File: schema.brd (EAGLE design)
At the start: 59.4 x 55.9 mm, 24 parts, among them Q1 2N2907

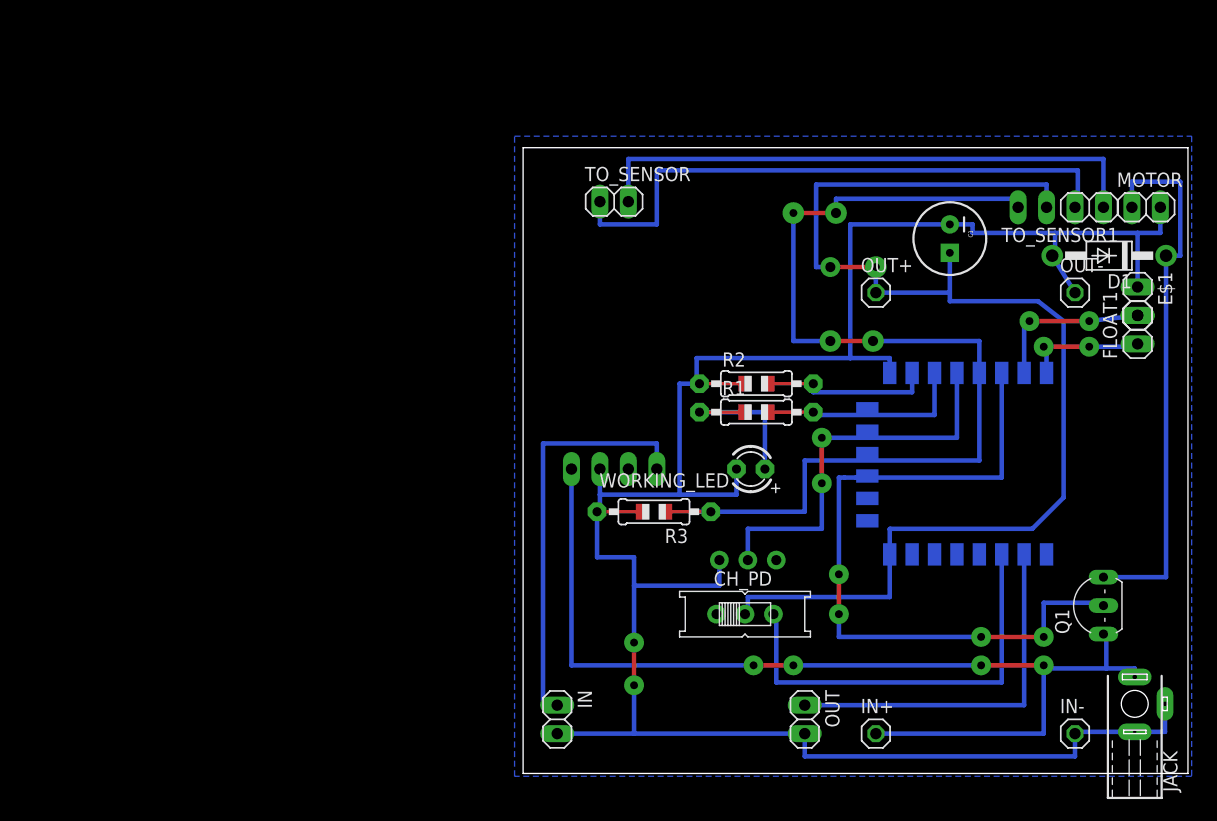
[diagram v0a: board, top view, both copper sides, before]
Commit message: Version 2
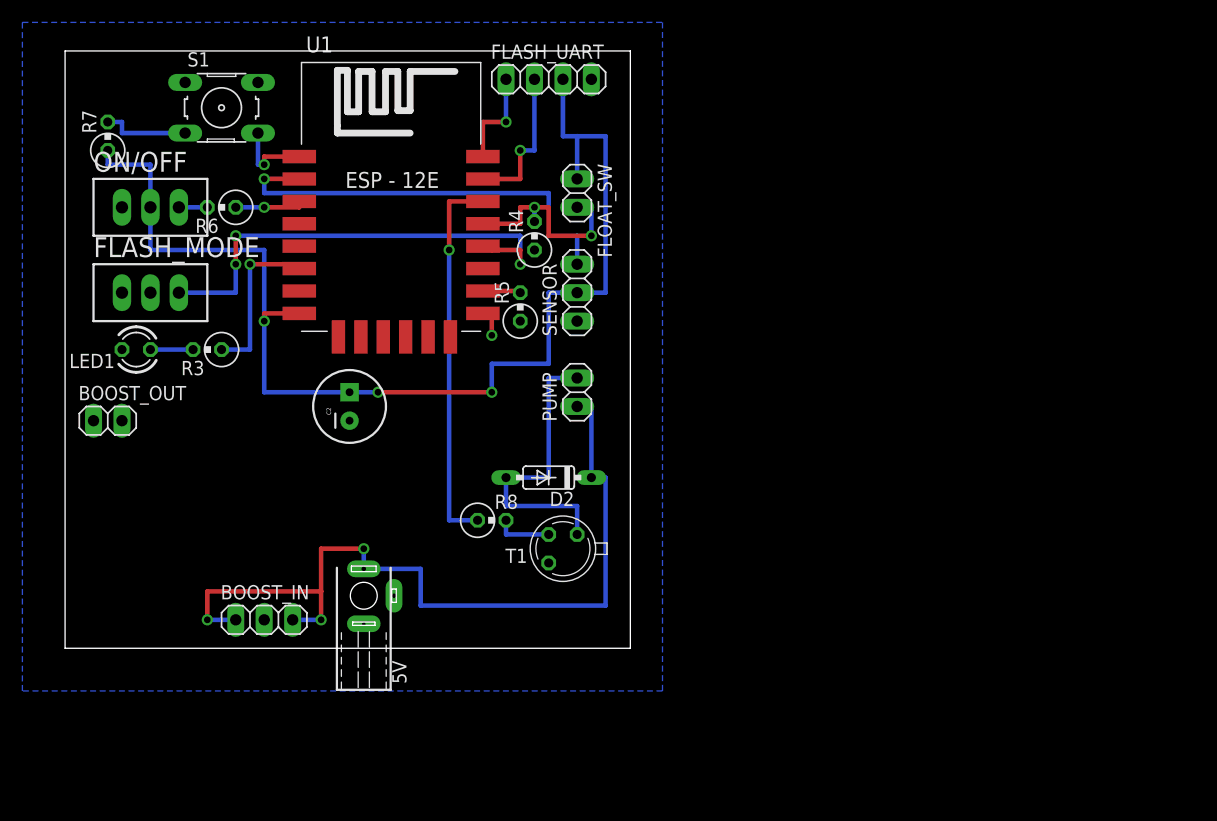
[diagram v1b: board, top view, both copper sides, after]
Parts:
- removed C1: 2200uF, SparkFun-Capacitors:CPOL-RADIAL-100UF-25V
- removed CH_PD, FLASH: OFF, adafruit:EG1218
- removed D1: 1N4004, adafruit:DO41-10
- removed E$1: (no value), pinhead:1X02
- removed FLOAT: 3.3v, pinhead:1X02
- removed FLOAT1: RX_TX, pinhead:1X02
- removed HUM_SENSOR: VCC_GND_D0_A0, pinhead:1X04
- removed IN, MOTOR, TO_SENSOR, TO_SENSOR1: 5V, pinhead:1X02
- removed IN+, IN-: 5v, pinhead:1X01
- removed JACK: 5V IN, con-conrad:733989-5
- removed MDL1: ESP-12, ESP8266-ESP12E:ESP8266-ESP12E
- removed OUT: 3.3V, pinhead:1X02
- removed OUT+, OUT-: 3.3v, pinhead:1X01
- removed Q1: 2N2907, adafruit:TO92-EBC-OVAL
- removed R1, R2: 300, adafruit:0805-THM
- removed WORKING_LED: 3.3v, adafruit:LED3MM
- added 5V: +5V, con-conrad:733989-5
- added BOOST_IN, SENSOR: (no value), pinhead:1X03
- added BOOST_OUT, FLOAT_SW, PUMP: (no value), pinhead:1X02
- added C2: 2200uF, SparkFun-Capacitors:CPOL-RADIAL-100UF-25V
- added D2: 1N4148DO35-7, diode:DO35-7
- added FLASH_MODE, ON/OFF: TL36PO, switch:TL3XPO
- added FLASH_UART: (no value), pinhead:1X04
- added LED1: WORK, led:LED3MM
- added R4, R5, R6, R7: 10k, resistor:0309V
- added R8: 220, resistor:0309V
- added S1: RST_SW, switch-omron:B3F-10XX
- added T1: 2N2222, transistor:TO18
- added U1: ESP12E, esp8266modules:ESP12E-SMD
- R3: device adafruit:0805-THM -> resistor:0309V
- moved R3 42.4 mm to (12.7, 34.3)
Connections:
- removed net N$1: HUM_SENSOR.4, IN.1
- removed net N$10: FLASH.P, MDL1.12
- removed net N$12: D1.C, MOTOR.1, Q1.C
- removed net N$13: FLOAT.1, MDL1.13, R3.1
- removed net N$2: MDL1.14, Q1.B
- removed net N$3: MDL1.11, R1.2
- removed net N$4: CH_PD.S, MDL1.3
- removed net N$5: FLOAT1.2, MDL1.15
- removed net N$6: MDL1.2, OUT.1
- removed net N$8: R1.1, WORKING_LED.A
- removed net N$9: MDL1.10, R2.2
- removed net S$1: TO_SENSOR.2, TO_SENSOR1.1
- removed net S$2: TO_SENSOR.1, TO_SENSOR1.2
- removed net SS: FLOAT1.1, MDL1.16
- new net ADC: SENSOR.3, U1.ADC
- new net CH_PD: R6.1, U1.CH_PD
- new net CH_PD_S: ON/OFF.3, R6.2
- new net GPIO0: FLASH_MODE.3, U1.GPIO0
- new net GPIO12: R3.1, U1.GPIO12
- new net GPIO12D: LED1.A, R3.2
- new net GPIO15: R5.2, U1.GPIO15
- new net GPIO4: FLOAT_SW.2, R4.2, U1.GPIO4
- new net GPIO5: R8.1, U1.GPIO5
- new net GPIO5_T: R8.2, T1.2
- new net PUMP_GND: D2.A, PUMP.2, T1.1
- new net RST: S1.4, U1.RESET
- new net RST_R: R7.2, S1.3
- new net RX: FLASH_UART.2, U1.RXD0
- new net TX: FLASH_UART.1, U1.TXD0
- net +3V3: now also BOOST_OUT.2, C2.1, FLASH_UART.3, FLOAT_SW.1, ON/OFF.2, R7.1, SENSOR.2, U1.VCC; no longer C1.1, CH_PD.P, FLOAT.2, MDL1.8, OUT+.1
- net +5V: now also 5V.1, BOOST_IN.1, BOOST_IN.3, D2.C, PUMP.1; no longer HUM_SENSOR.1, IN+.1, JACK.1, Q1.E
- net GND: now also 5V.2, 5V.3, BOOST_IN.2, BOOST_OUT.1, C2.2, FLASH_MODE.2, FLASH_UART.4, LED1.K, R4.1, R5.1, S1.1, S1.2, SENSOR.1, T1.3, U1.GND; no longer C1.2, D1.A, E$1.1, FLASH.S, HUM_SENSOR.2, IN-.1, IN.2, JACK.2, JACK.3, MDL1.9, MOTOR.2, OUT-.1, OUT.2, R2.1, R3.2, WORKING_LED.K
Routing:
- net GND: track 199.0 -> 2.75 mm, vias 2 -> 1
- net N$13: track 90.6 -> 0.00 mm, vias 4 -> 0
- net N$2: track 65.0 -> 0.00 mm, vias 4 -> 0
- net S$2: track 53.1 -> 0.00 mm
- net S$1: track 50.5 -> 0.00 mm
- net N$12: track 48.8 -> 0.00 mm
- net GPIO0: track 0.00 -> 43.4 mm, vias 0 -> 3
- net ADC: track 0.00 -> 38.7 mm, vias 0 -> 1
- net N$4: track 37.9 -> 0.00 mm
- net N$1: track 37.1 -> 0.00 mm
- net N$10: track 35.4 -> 0.00 mm, vias 2 -> 0
- net GPIO5: track 0.00 -> 34.0 mm, vias 0 -> 1
- net N$6: track 33.0 -> 0.00 mm
- net PUMP_GND: track 0.00 -> 26.7 mm
- net GPIO4: track 0.00 -> 18.8 mm, vias 0 -> 2
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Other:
- board size 59.4 x 55.9 mm -> 50.5 x 53.3 mm
